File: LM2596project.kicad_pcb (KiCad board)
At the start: 2 copper layers, 56.1 x 32.9 mm, 15 parts, among them J1 Screw_Terminal_01x02, J2 Screw_Terminal_01x02, U1 LM2596S-ADJ

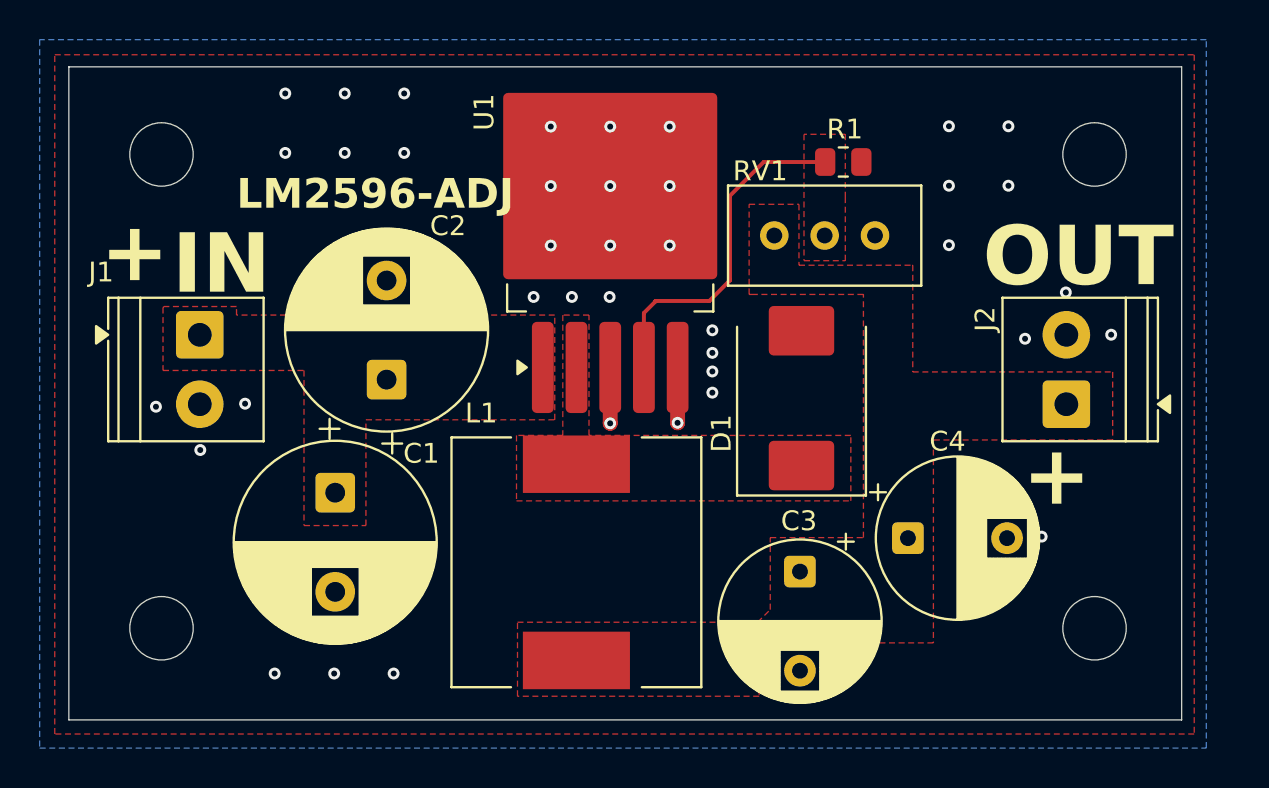
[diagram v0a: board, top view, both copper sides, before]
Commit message: Add files via upload
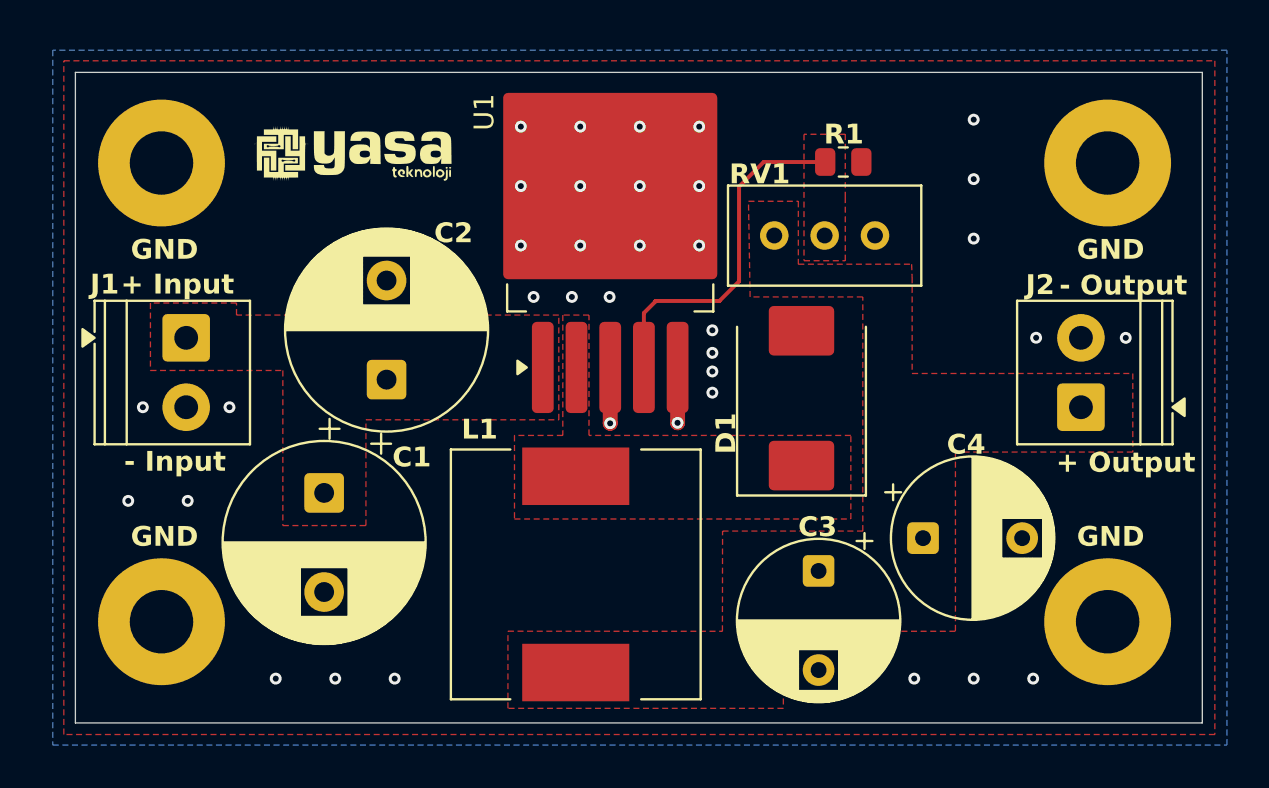
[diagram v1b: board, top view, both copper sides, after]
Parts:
- removed the REF** at (27.1, 122.8)
- removed the REF** at (74.1, 146.7)
- removed the REF** at (27.1, 146.7)
- removed the REF** at (74.1, 122.8)
- added G***: LOGO, LOGO, F.Cu at (36.7, 122.8)
- added G***: LOGO, LOGO, B.Cu at (50.9, 137.7)
- added REF**: MountingHole_3.2mm_M3_Pad, MountingHole:MountingHole_3.2mm_M3_Pad, F.Cu at (74.8, 123.2)
- added REF**: MountingHole_3.2mm_M3_Pad, MountingHole:MountingHole_3.2mm_M3_Pad, F.Cu at (27.1, 123.2)
- added REF**: MountingHole_3.2mm_M3_Pad, MountingHole:MountingHole_3.2mm_M3_Pad, F.Cu at (27.1, 146.4)
- added REF**: MountingHole_3.2mm_M3_Pad, MountingHole:MountingHole_3.2mm_M3_Pad, F.Cu at (74.8, 146.4)
- moved C3 0.94 mm to (60.2, 143.8)
- moved C4 0.76 mm to (65.5, 142.2)
- moved J2 0.75 mm to (73.4, 135.6)
- moved J1 0.70 mm to (28.3, 132.1)
- moved L1 0.61 mm to (48.0, 144.0)
- moved C1 0.56 mm to (35.3, 139.9)
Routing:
- net GND: vias 50 -> 55
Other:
- board size 56.1 x 32.9 mm -> 56.8 x 32.8 mm
- board text added: "+ Input"
- board text added: "+ Output"
- board text added: "-"
- board text added: "- Input"
- board text added: "- Output"
- board text added: "GND"
- board text added: "Input"
- board text added: "Output"
- board text removed: "IN"
- board text removed: "LM2596-ADJ"
- board text removed: "OUT"
